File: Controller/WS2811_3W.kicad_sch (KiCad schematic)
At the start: 19 parts, among them J1 Conn_01x01_Female, J2 Conn_01x01_Female, J3 Conn_01x01_Female, J4 Conn_01x01_Female, J5 Conn_01x01_Female, J6 Conn_01x01_Female, U1 MAX485E, U2 WS2811, U3 MAX485E, U4 AMS1117-5.0

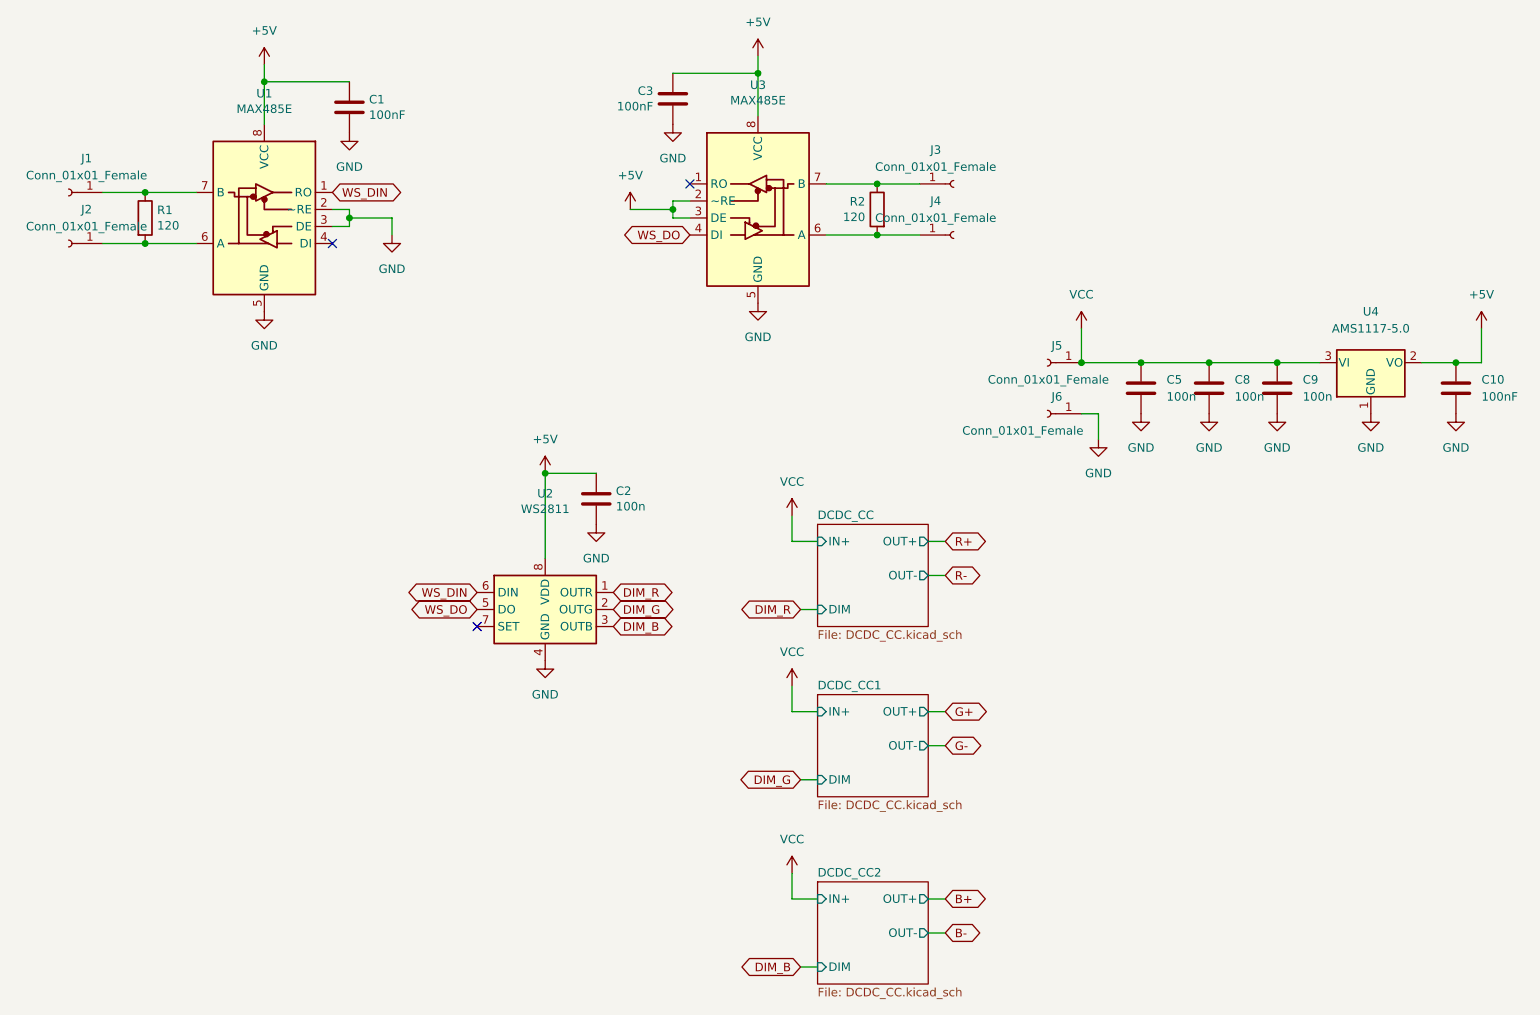
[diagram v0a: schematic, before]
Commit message: pcb stuff
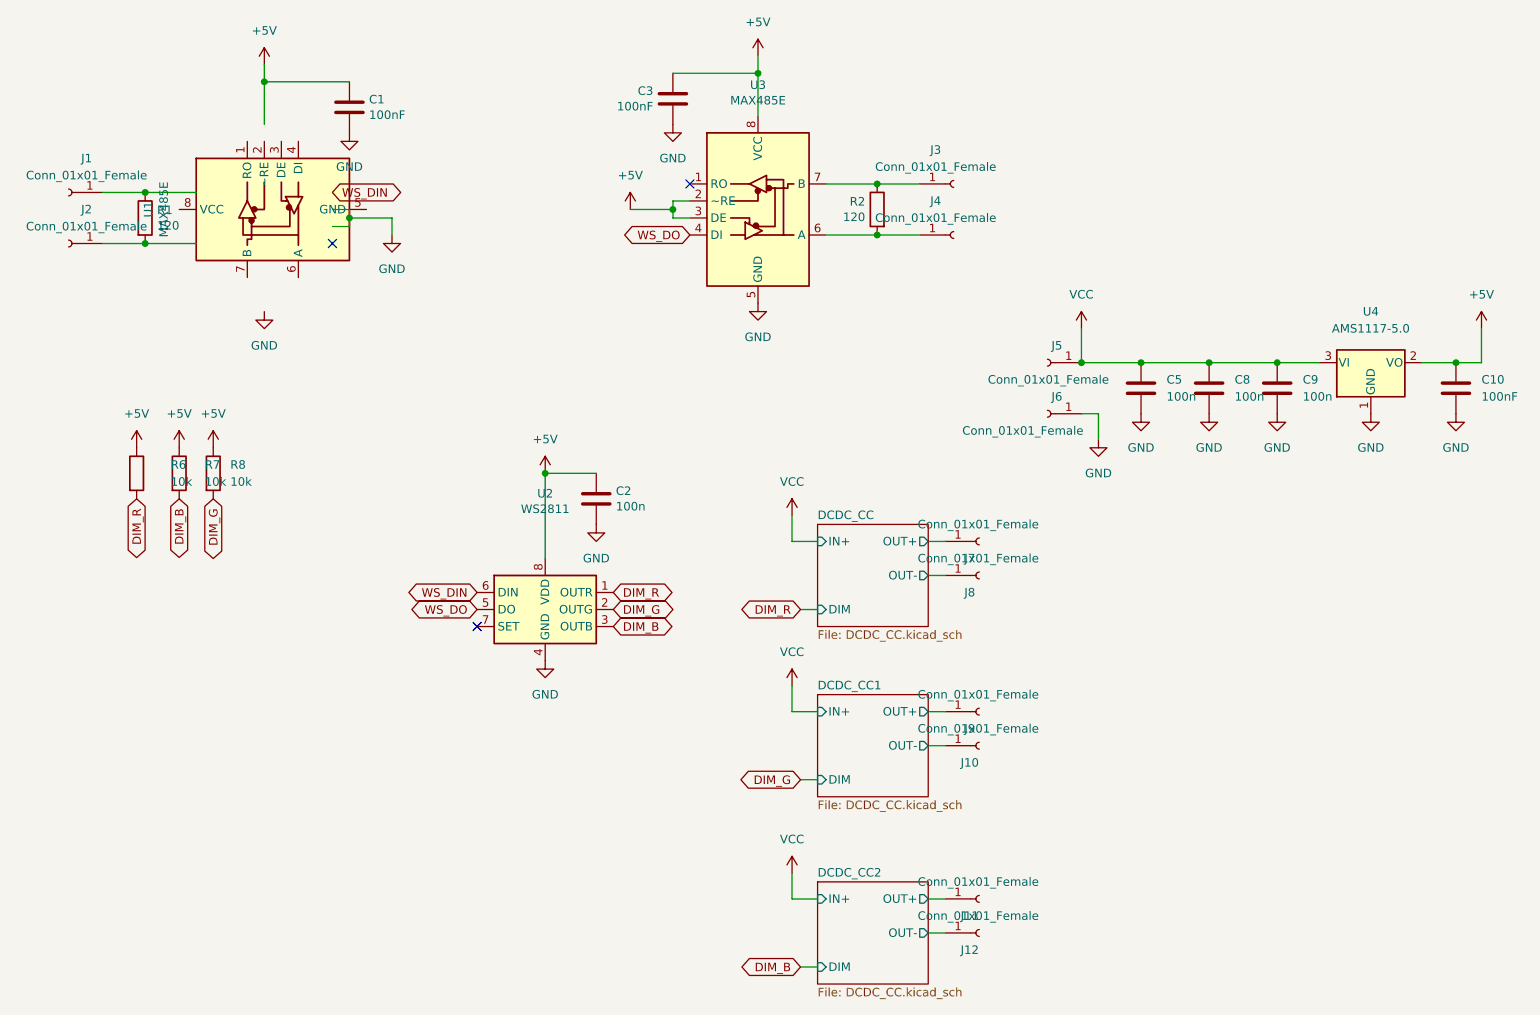
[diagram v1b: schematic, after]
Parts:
- added J10, J11, J12, J7, J8, J9: Conn_01x01_Female, Connector_Wire:SolderWirePad_1x01_SMD_1x2mm, symbol Connector:Conn_01x01_Female
- added R6, R7, R8: 10k, Resistor_SMD:R_0603_1608Metric, symbol Device:R
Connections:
- net +5V: now also R6.1, R7.1, R8.1; no longer U1.8 (VCC)
- net DIM_B: now also R7.2
- net DIM_G: now also R8.2
- net DIM_R: now also R6.2
- net GND: no longer U1.2 (~RE), U1.3 (DE), U1.5 (GND)
- net WS_DIN: no longer U1.1 (RO)
- net at J2.1 (Pin_1), R1.2: no longer U1.6 (A)
- net at J1.1 (Pin_1), R1.1: no longer U1.7 (B)
- new net DCDC_CC/OUT+: J7.1 (Pin_1)
- new net DCDC_CC/OUT-: J8.1 (Pin_1)
- new net DCDC_CC1/OUT+: J9.1 (Pin_1)
- new net DCDC_CC1/OUT-: J10.1 (Pin_1)
- new net DCDC_CC2/OUT+: J11.1 (Pin_1)
- new net DCDC_CC2/OUT-: J12.1 (Pin_1)
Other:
- moved on the sheet: U1
